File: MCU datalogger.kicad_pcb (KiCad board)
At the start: 2 copper layers, 50.8 x 30.5 mm, 29 parts, among them J1 Conn_01x04_Pin, J2 Conn_01x04_Pin, J3 Conn_01x09_Pin, J4 Conn_02x03_Odd_Even, U1 24LC1025, U2 24LC1025, U3 DS1337S_, U4 ATMEGA328P-AU, Y1 32.768 KHz, Y2 16 MHz

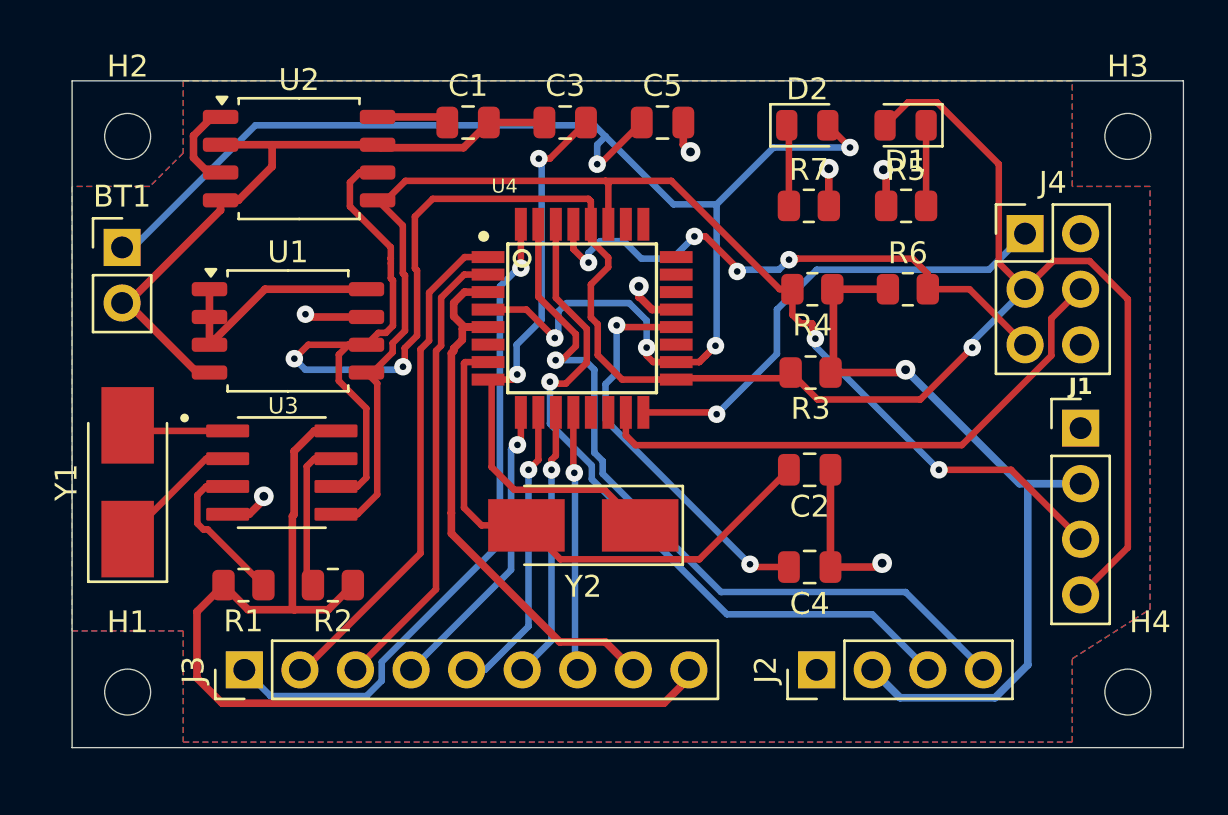
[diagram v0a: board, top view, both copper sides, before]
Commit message: Completed Design of 2-layer
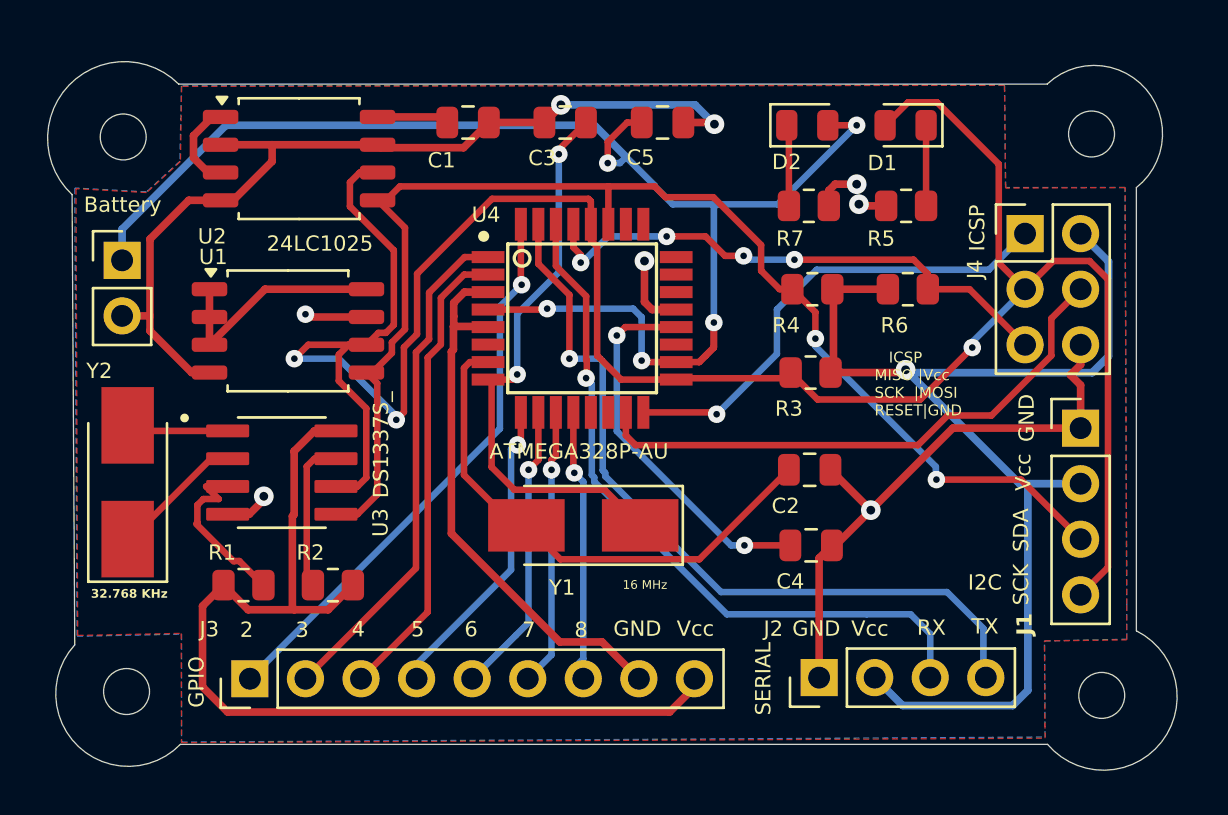
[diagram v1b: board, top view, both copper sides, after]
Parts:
- moved H3 1.66 mm to (110.1, 88.8)
- moved H4 1.20 mm to (110.6, 114.5)
- moved C4 0.99 mm to (97.3, 107.6)
- moved BT1 0.59 mm to (65.8, 94.6)
- moved J3 0.48 mm to (71.6, 113.7)
- moved J2 0.37 mm to (97.6, 113.6)
- moved H2 0.20 mm to (65.8, 88.9)
- moved H1 0.06 mm to (66.0, 114.3)
- renumbered Y2 to Y1, Y1 to Y2
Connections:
- BT1 pad 1: Net-(BT1-+) -> /Vcc
- C5 pad 1: Net-(BT1-+) -> /Vcc
- D2 pad 2: Net-(BT1-+) -> /Vcc
- U4 pad 18: Net-(BT1-+) -> /Vcc
- U4 pad 4: Net-(BT1-+) -> /Vcc
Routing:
- net /Vcc: track 100.6 -> 184.4 mm, vias 1 -> 6
- net Net-(BT1-+): track 66.2 -> 0.00 mm, vias 5 -> 0
- net GND: track 76.8 -> 105.9 mm, vias 7 -> 8
- net /D2: track 30.6 -> 25.8 mm
- net /RESET: track 26.5 -> 25.2 mm
- net Net-(U4-AREF): track 18.5 -> 17.3 mm
- net Net-(U4-PB6): track 25.3 -> 24.2 mm
- net Net-(U3-~{INTA}): track 7.03 -> 7.88 mm
- net Net-(U4-PB7): track 26.7 -> 26.2 mm
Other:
- board size 50.8 x 30.5 mm -> 51.6 x 32.4 mm
- board text added: "2"
- board text added: "2Mbit EEPROM RTC I2C, SPI, GPIO's"
- board text added: "3"
- board text added: "4"
- board text added: "5"
- board text added: "6"
- board text added: "7"
- board text added: "8"
- board text added: "Data Logger with ATMega328P."
- board text added: "GND"
- board text added: "GPIO"
- board text added: "I2C"
- board text added: "ICSP"
- board text added: "ICSP MISO |Vcc SCK |MOSI RESET|GND"
- board text added: "RX"
- board text added: "SCK"
- board text added: "SDA"
- board text added: "SERIAL"
- board text added: "TX"
- board text added: "Vcc"
